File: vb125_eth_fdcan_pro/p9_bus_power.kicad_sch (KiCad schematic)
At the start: 13 parts, among them U7 LT8304IS8E#PBF

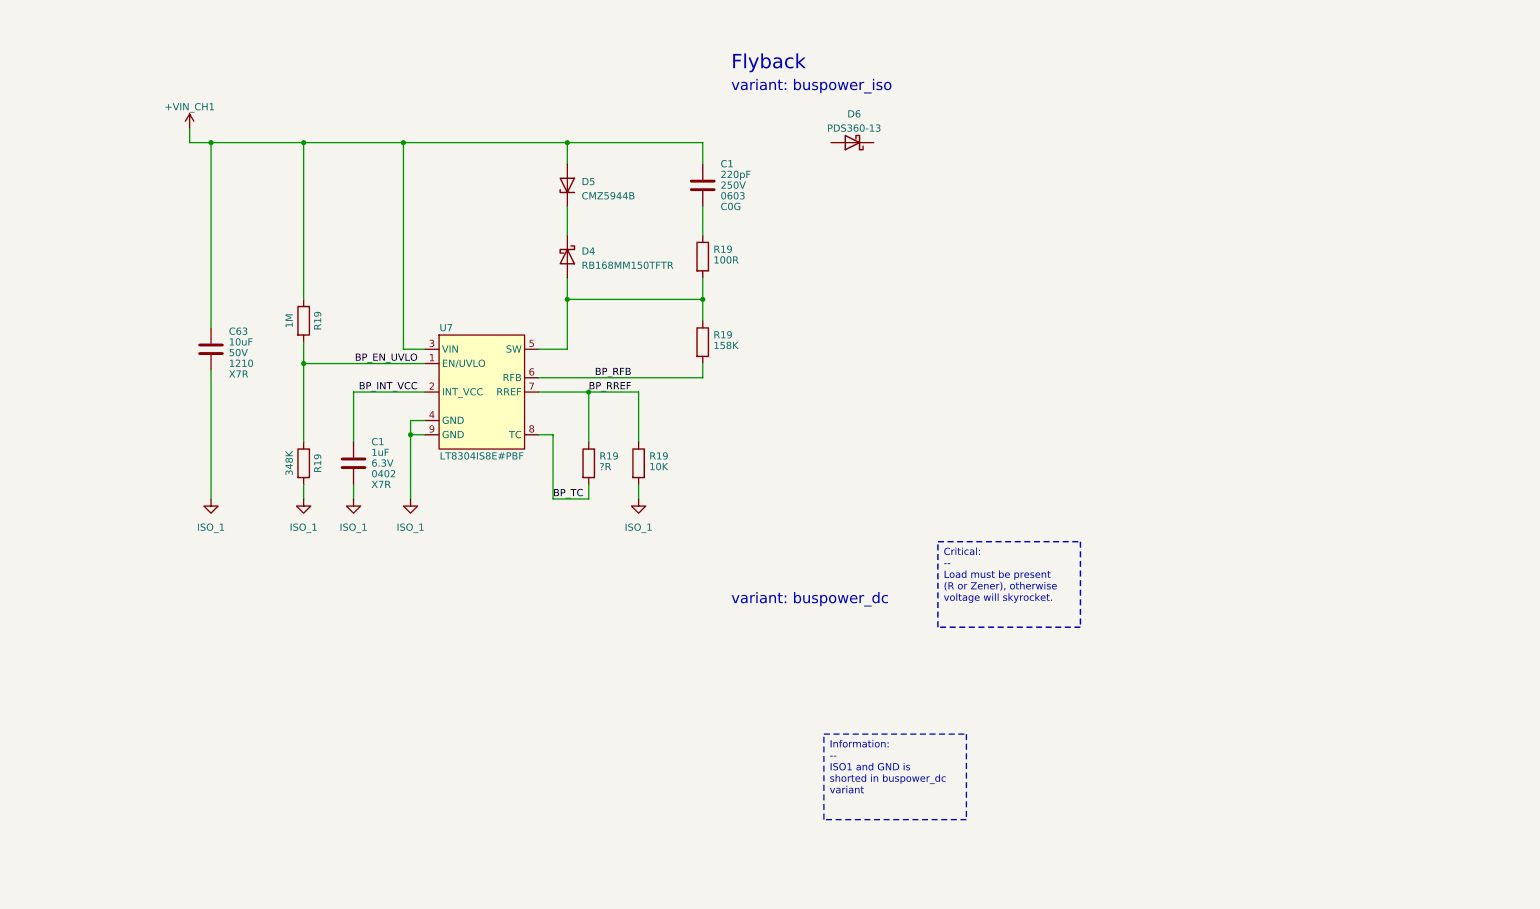
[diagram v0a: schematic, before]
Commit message: Finish schematics.
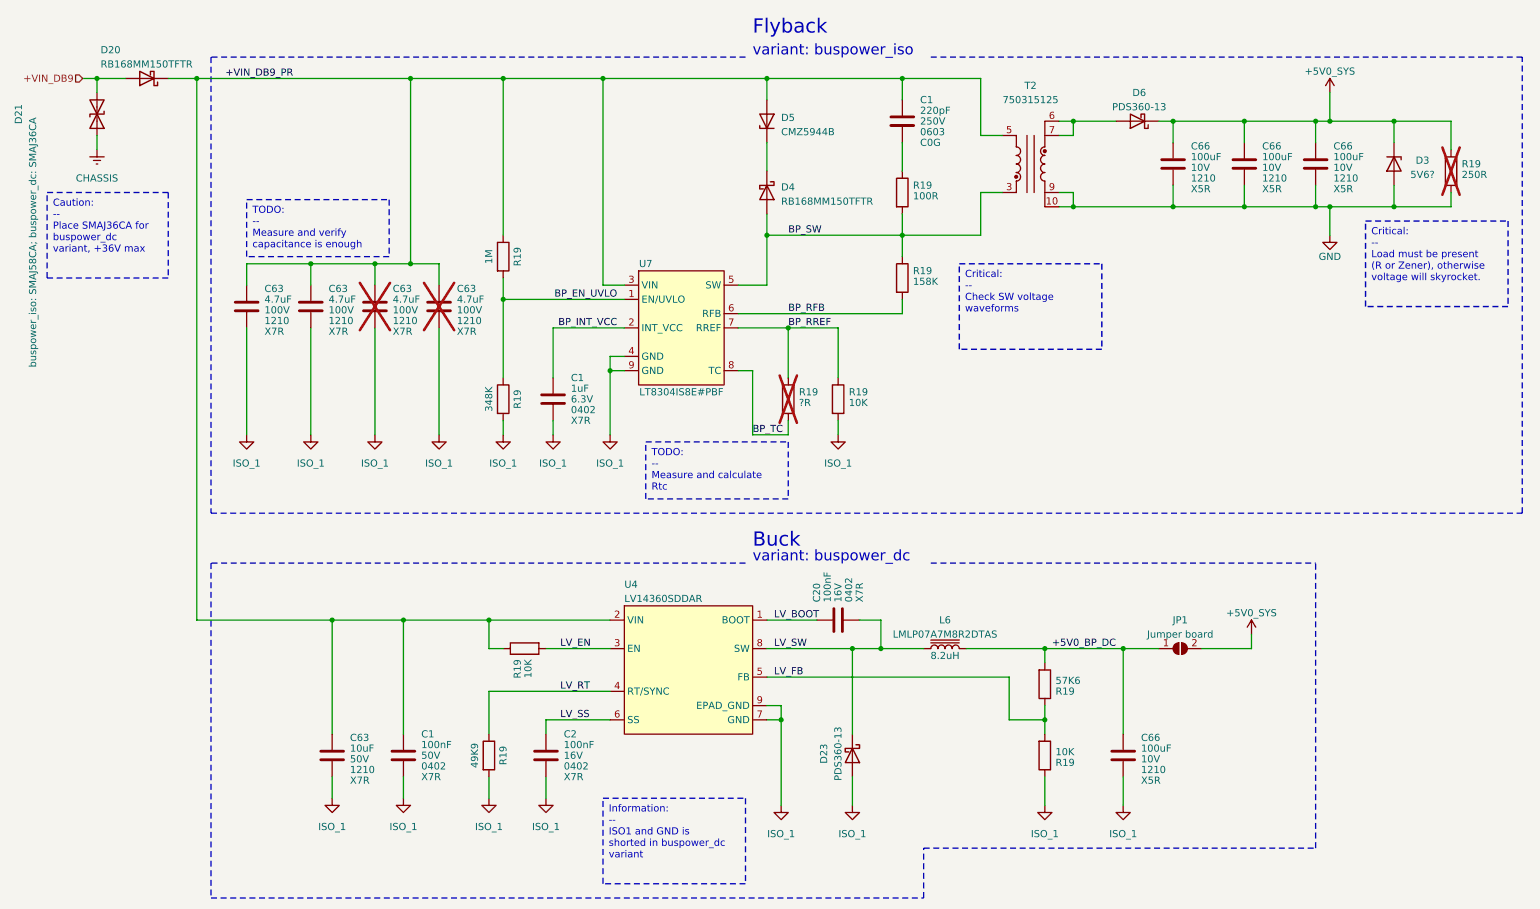
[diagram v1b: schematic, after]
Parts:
- added C1, C2, C20: 100nF, Capacitor_SMD:C_0402_1005Metric, symbol Device:C
- added C63 (x4): 4.7uF, Capacitor_SMD:C_1210_3225Metric, symbol Device:C
- added C66 (x4): 100uF, Capacitor_SMD:C_1210_3225Metric, symbol Device:C
- added D20: RB168MM150TFTR, Diode_SMD:D_SOD-123F, symbol Device:D_Schottky
- added D21: buspower_iso: SMAJ58CA; buspower_dc: SMAJ36CA, Diode_SMD:D_SMA, symbol Device:D_TVS
- added D23: PDS360-13, Diode_SMD:D_PowerDI-5, symbol Device:D_Schottky
- added D3: 5V6?, Diode_SMD:D_SOD-323, symbol Device:D_Zener
- added JP1: Jumper board, vhrd_generic:PCB_JUMPER, symbol Jumper:SolderJumper_2_Open
- added L6: LMLP07A7M8R2DTAS, vhrd_inductor:LMLP07A7, symbol Device:L_Iron
- added R19 (x2): 10K, Resistor_SMD:R_0402_1005Metric, symbol Device:R
- added R19: 250R, Resistor_SMD:R_0603_1608Metric, symbol Device:R
- added R19: 57K6, Resistor_SMD:R_0402_1005Metric, symbol Device:R
- added R19: 49K9, Resistor_SMD:R_0402_1005Metric, symbol Device:R
- added T2: 750315125, vhrd_transformer:750315125, symbol vhrd_transformer:750315125
- added U4: LV14360SDDAR, Package_SO:SOIC-8-1EP_3.9x4.9mm_P1.27mm_EP2.95x4.9mm_Mask2.71x3.4mm_ThermalVias, symbol vhrd_pmic_regulator:LV14360SDDAR
- C1: footprint (none) -> Capacitor_SMD:C_0603_1608Metric
- C1: footprint (none) -> Capacitor_SMD:C_0402_1005Metric
- D6: Irated (none) -> 3A; Vrated (none) -> 60V
- R19: now not fitted
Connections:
- net ISO_1: now also C1.2, C2.2, C63.2, C63.2, C63.2, C63.2, C66.2, D23.2 (A), R19.1, R19.2, U4.7 (GND), U4.9 (EPAD_GND)
- net BP_SW: now reaches D4.2 (A), R19.1, R19.2, U7.5 (SW)
- net BP_SW: now also T2.3
- net +5V0_SYS: now reaches D6.1 (K)
- net +5V0_SYS: now also C66.1, C66.1, C66.1, D3.1 (K), JP1.2 (B), R19.1
- net at D6.2 (A): now also T2.6, T2.7
- net +VIN_CH1 renamed +VIN_DB9_PR
- net +VIN_DB9_PR: now also C1.1, C63.1, C63.1, C63.1, C63.1, D20.1 (K), R19.1, T2.5, U4.2 (VIN)
- new net +5V0_BP_DC: C66.1, JP1.1 (A), L6.2, R19.2
- new net +VIN_DB9: D20.2 (A), D21.2 (A2)
- new net CHASSIS: D21.1 (A1)
- new net GND: C66.2, C66.2, C66.2, D3.2 (A), R19.2, T2.10, T2.9
- new net LV_BOOT: C20.1, U4.1 (BOOT)
- new net LV_EN: R19.2, U4.3 (EN)
- new net LV_FB: R19.1, R19.2, U4.5 (FB)
- new net LV_RT: R19.1, U4.4 (RT/SYNC)
- new net LV_SS: C2.1, U4.6 (SS)
- new net LV_SW: C20.2, D23.1 (K), L6.1, U4.8 (SW)
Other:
- note added: "Buck"
- moved on the sheet: C1, C63, D4, D5, D6, R19, U7
